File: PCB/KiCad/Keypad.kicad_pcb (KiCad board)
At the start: 2 copper layers, 77 x 132.8 mm, 17 parts, among them SW1 SW_SPDT, U1 TP4056, U2 MT3608, U3 WeMos_D1_mini

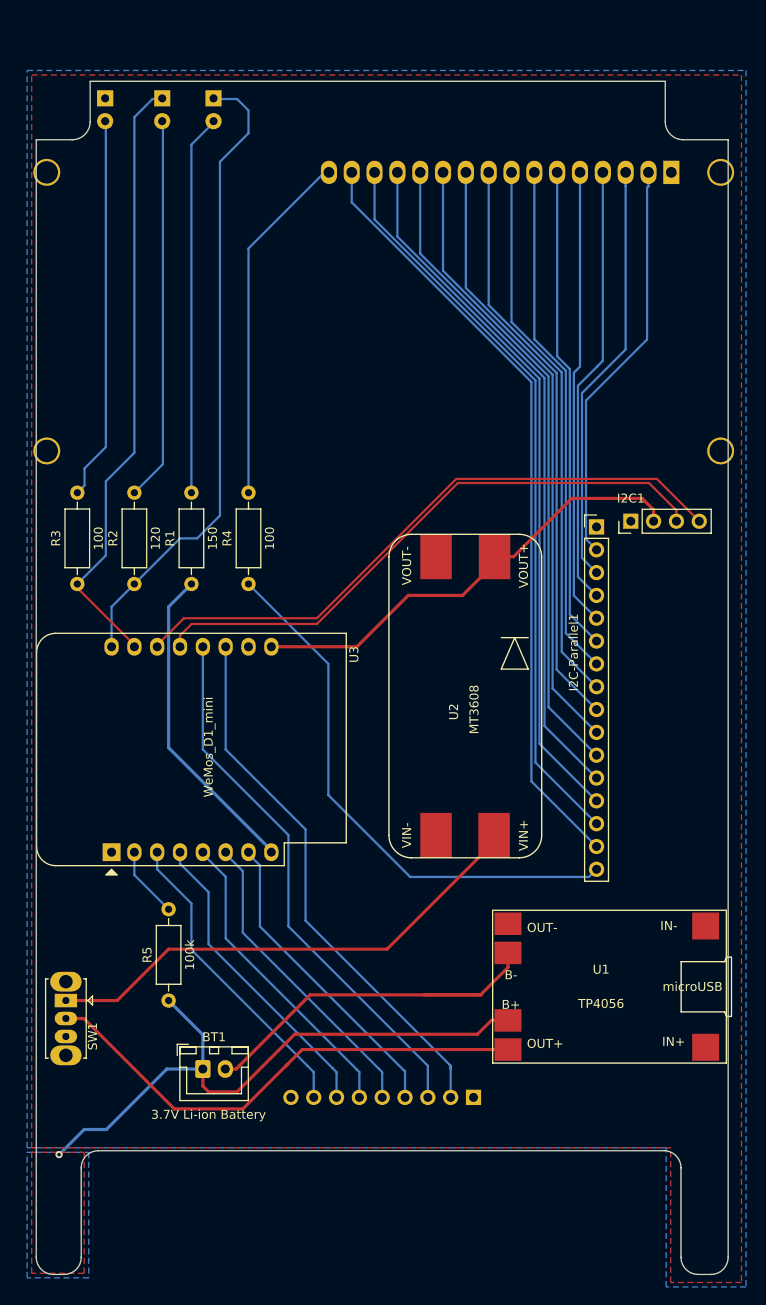
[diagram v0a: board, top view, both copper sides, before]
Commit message: kicad files updated.
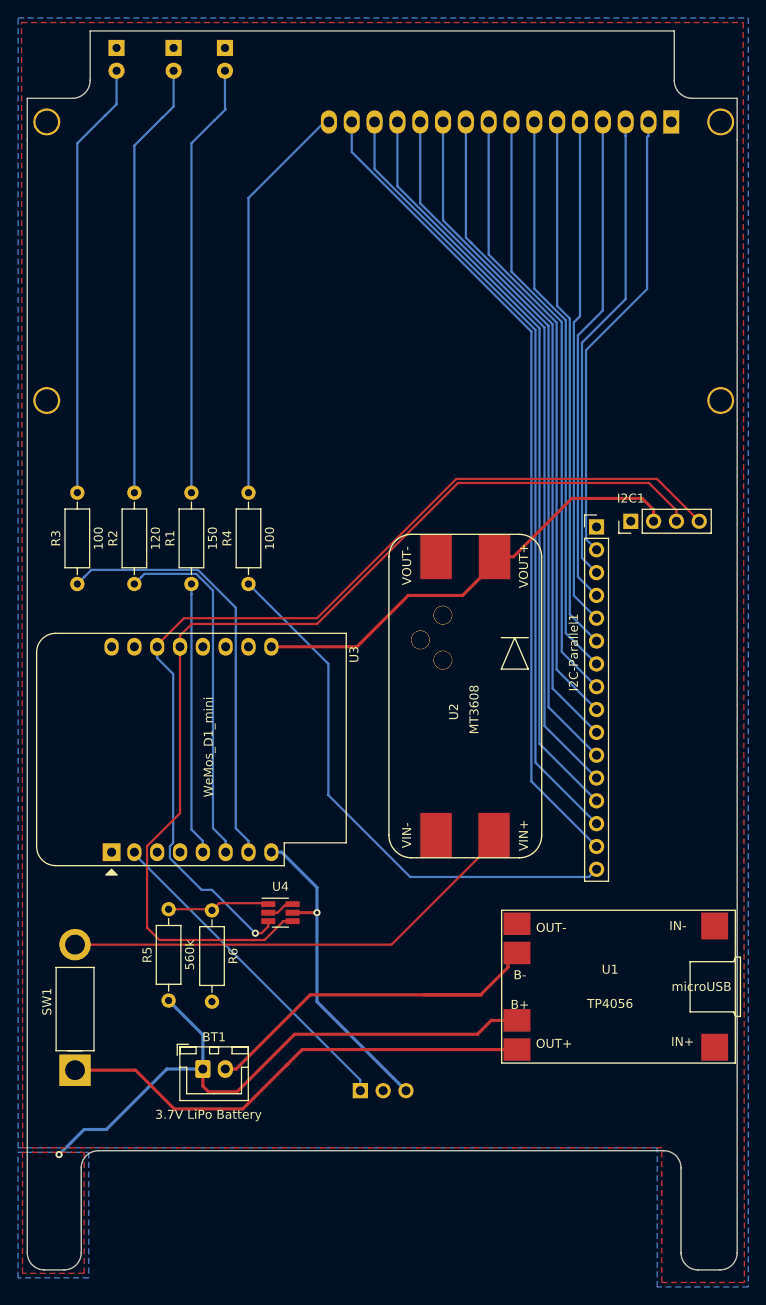
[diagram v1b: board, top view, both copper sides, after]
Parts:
- added R6: 500K, Resistor_THT:R_Axial_DIN0207_L6.3mm_D2.5mm_P10.16mm_Horizontal, F.Cu at (130.6, 127.8)
- added U4: MCP3421A0T-ECH, Package_TO_SOT_SMD:SOT-23-6_Handsoldering, F.Cu at (138.2, 128.0)
- BT1: value 3.7V Li-ion Battery -> 3.7V LiPo Battery
- Keypad1: value Conn_01x09 -> Conn_01x03; footprint Connector_PinHeader_2.54mm:PinHeader_1x09_P2.54mm_Vertical -> Connector_PinHeader_2.54mm:PinHeader_1x03_P2.54mm_Vertical
- R5: value 100k -> 560k
- SW1: value SW_SPDT -> SW_DIP_x01; footprint Button_Switch_THT:SW_Slide_1P2T_CK_OS102011MS2Q -> Keypad:Mini_Latching_Torch_Switch
- moved Keypad1 12.6 mm to (147.1, 147.8), turned to 270 degrees
- moved SW1 7.81 mm to (115.3, 145.5), turned to 90 degrees
- moved D1 5.75 mm to (132.0, 31.8)
- moved D2 5.75 mm to (126.3, 31.8)
- moved D3 5.75 mm to (119.9, 31.8)
- moved DS1 5.61 mm to (181.7, 40.0)
- moved U1 1.00 mm to (175.5, 136.2)
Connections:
- D1 pad 1: /LED_Control1 -> GND
- D2 pad 1: /LED_Control2 -> GND
- Keypad1 pad 1: Net-(Keypad1-Pad1) -> keypad
- Keypad1 pad 2: /KP1 -> GND
- Keypad1 pad 3: /KP2 -> +3V3
- R1 pad 1: +3V3 -> red
- R2 pad 1: /LED_Control1 -> yellow
- R3 pad 1: /LED_Control2 -> green
- SW1 pad 1: /V+2 -> /V+1
- SW1 pad 2: /V+1 -> Net-(SW1-Pad2)
- U2 pad 1: /V+2 -> Net-(SW1-Pad2)
- U3 pad 11: /KP1 -> Net-(U3-Pad11)
- U3 pad 12: /KP2 -> Net-(U3-Pad12)
- U3 pad 15: /LED_Control2 -> Net-(U3-Pad15)
- U3 pad 16: /LED_Control1 -> Net-(U3-Pad16)
- U3 pad 2: Net-(R5-Pad2) -> keypad
- U3 pad 3: /KP7 -> Net-(U3-Pad3)
- U3 pad 4: /KP6 -> Net-(U3-Pad4)
- U3 pad 5: /KP5 -> red
- U3 pad 6: /KP4 -> yellow
- U3 pad 7: /KP3 -> green
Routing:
- net /LED_Control1: track 71.5 -> 0.00 mm
- net /LED_Control2: track 68.2 -> 0.00 mm
- net /KP1: track 61.0 -> 0.00 mm
- net /KP2: track 60.5 -> 0.00 mm
- net /V+2: track 55.7 -> 0.00 mm
- net Net-(SW1-Pad2): track 0.00 -> 53.1 mm
- net SDA: track 66.0 -> 116.4 mm
- net green: track 0.00 -> 48.5 mm
- net yellow: track 0.00 -> 39.9 mm
- net SCL: track 70.1 -> 109.8 mm, vias 0 -> 1
- net keypad: track 0.00 -> 37.0 mm
- net /KP7: track 34.5 -> 0.00 mm
- net /KP6: track 34.5 -> 0.00 mm
- net /KP4: track 34.5 -> 0.00 mm
- net /KP3: track 34.5 -> 0.00 mm
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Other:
- board size 77 x 132.8 mm -> 79 x 137.9 mm
